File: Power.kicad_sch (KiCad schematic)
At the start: 23 parts, among them IC1 SC4216HSETRT, J4 Conn_01x03, J5 Conn_01x02, U8 TPS62933P

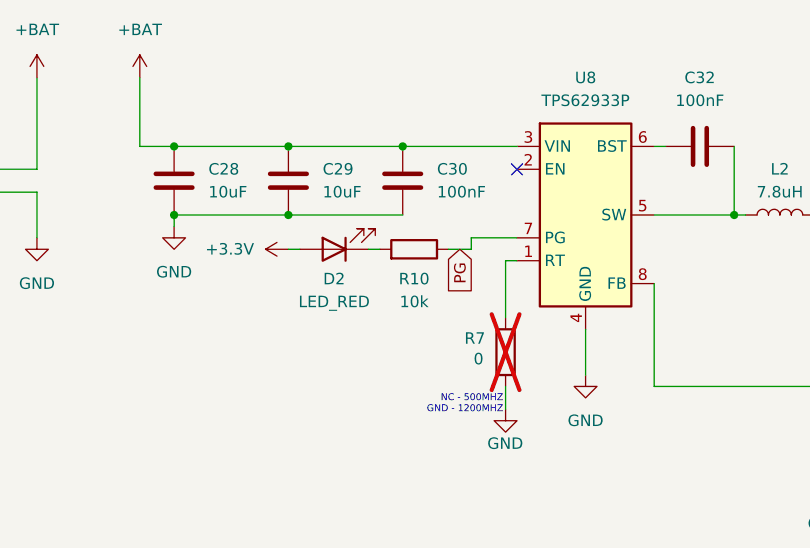
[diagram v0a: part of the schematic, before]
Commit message: "Update KiRA Flight Computer schematic and PCB files"
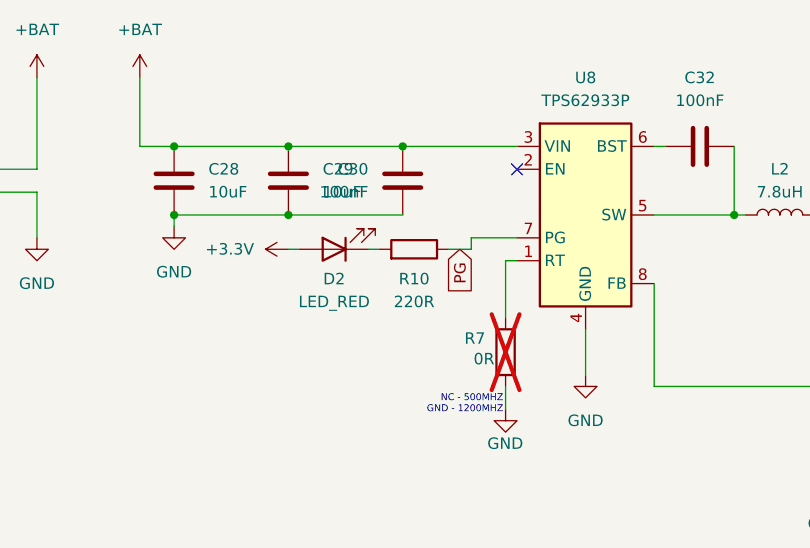
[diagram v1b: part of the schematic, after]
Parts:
- C28: footprint (none) -> Capacitor_SMD:C_1206_3216Metric; Source (none) -> https://www.lcsc.com/product-detail/C89632.html
- C29, C34, C35: footprint (none) -> Capacitor_SMD:C_1206_3216Metric
- C30: footprint (none) -> Capacitor_SMD:C_0603_1608Metric; Source (none) -> https://www.lcsc.com/product-detail/C1591.html
- C31: footprint (none) -> Capacitor_SMD:C_1210_3225Metric
- C32, C36: footprint (none) -> Capacitor_SMD:C_0603_1608Metric
- C33: footprint (none) -> Capacitor_SMD:C_0603_1608Metric; Source (none) -> https://www.lcsc.com/product-detail/C69335.html
- D2, D3: footprint (none) -> LED_SMD:LED_0603_1608Metric
- IC1: footprint SOIC127P600X175-9N -> dep:SOIC127P600X175-9N
- J4: footprint (none) -> Connector_PinSocket_2.54mm:PinSocket_1x03_P2.54mm_Vertical
- J5: footprint (none) -> Connector_AMASS:AMASS_XT30U-F_1x02_P5.0mm_Vertical
- L2: footprint (none) -> dep:Inductor 60A782C
- R10: value 10k -> 220R; footprint (none) -> Resistor_SMD:R_0402_1005Metric
- R11: footprint (none) -> Resistor_SMD:R_0402_1005Metric
- R12, R8: footprint (none) -> Resistor_SMD:R_0805_2012Metric
- R13, R9: footprint (none) -> Resistor_SMD:R_0603_1608Metric
- R7: value 0 -> 0R; footprint (none) -> Resistor_SMD:R_0603_1608Metric
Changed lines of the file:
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@@
 			)
 		)
-		(property "Footprint" ""
+		(property "Footprint" "LED_SMD:LED_0603_1608Metric"
 			(at 228.6 87.63 0)
 			(effects
@@
 			)
 		)
-		(property "Footprint" ""
+		(property "Footprint" "Connector_AMASS:AMASS_XT30U-F_1x02_P5.0mm_Vertical"
 			(at 21.59 78.74 0)
 			(effects
@@
 			)
 		)
-		(property "Footprint" ""
+		(property "Footprint" "Connector_PinSocket_2.54mm:PinSocket_1x03_P2.54mm_Vertical"
 			(at 200.66 81.28 0)
 			(effects
@@
 			)
 		)
-		(property "Footprint" ""
+		(property "Footprint" "Resistor_SMD:R_0805_2012Metric"
 			(at 106.172 135.89 90)
 			(effects
@@
 			)
 		)
-		(property "Footprint" ""
+		(property "Footprint" "Capacitor_SMD:C_1210_3225Metric"
 			(at 138.1252 96.52 0)
 			(effects
@@
 			)
 		)
-		(property "Footprint" ""
+		(property "Footprint" "Resistor_SMD:R_0603_1608Metric"
 			(at 106.172 146.05 90)
 			(effects
@@
 			)
 		)
-		(property "Footprint" ""
+		(property "Footprint" "dep:Inductor 60A782C"
 			(at 119.38 81.28 0)
 			(effects
@@
 			)
 		)
-		(property "Footprint" ""
+		(property "Footprint" "Capacitor_SMD:C_1206_3216Metric"
 			(at 53.0352 81.28 0)
 			(effects
@@
 			)
 		)
+		(property "Source" "https://www.lcsc.com/product-detail/C89632.html"
+			(at 52.07 77.47 0)
+			(effects
+				(font
+					(size 1.27 1.27)
+				)
+				(hide yes)
+			)
+		)
 		(pin "1"
 		)
@@
 			)
 		)
-		(property "Footprint" ""
+		(property "Footprint" "LED_SMD:LED_0603_1608Metric"
 			(at 69.85 85.09 0)
 			(effects
@@
 			)
 		)
-		(property "Footprint" "SOIC127P600X175-9N"
+		(property "Footprint" "dep:SOIC127P600X175-9N"
 			(at 87.63 230.81 0)
 			(effects
@@
 			)
 		)
-		(property "Footprint" ""
+		(property "Footprint" "Resistor_SMD:R_0603_1608Metric"
 			(at 122.682 105.41 90)
 			(effects
@@
 			)
 		)
-		(property "Footprint" ""
+		(property "Footprint" "Capacitor_SMD:C_1206_3216Metric"
 			(at 40.3352 148.59 0)
 			(effects
@@
 			)
 		)
-		(property "Footprint" ""
+		(property "Footprint" "Capacitor_SMD:C_0603_1608Metric"
 			(at 114.3 72.6948 0)
 			(effects
@@
 			)
 		)
-		(property "Footprint" ""
+		(property "Footprint" "Capacitor_SMD:C_0603_1608Metric"
 			(at 51.7652 148.59 0)
 			(effects
@@
 		)
 		(property "Description" "Unpolarized capacitor"
+			(at 50.8 144.78 0)
+			(effects
+				(font
+					(size 1.27 1.27)
+				)
+				(hide yes)
+			)
+		)
+		(property "Source" "https://www.lcsc.com/product-detail/C69335.html"
 			(at 50.8 144.78 0)
 			(effects
@@
 			)
 		)
-		(property "Footprint" ""
+		(property "Footprint" "Resistor_SMD:R_0402_1005Metric"
 			(at 226.822 95.25 90)
 			(effects
@@
 			)
 		)
-		(property "Value" "0"
+		(property "Value" "0R"
 			(at 85.344 97.282 0)
 			(effects
@@
 			)
 		)
-		(property "Footprint" ""
+		(property "Footprint" "Resistor_SMD:R_0603_1608Metric"
 			(at 87.122 96.52 90)
 			(effects
@@
 			)
 		)
-		(property "Footprint" ""
+		(property "Footprint" "Capacitor_SMD:C_1206_3216Metric"
 			(at 65.7352 81.28 0)
 			(effects
@@
 			)
 		)
-		(property "Footprint" ""
+		(property "Footprint" "Capacitor_SMD:C_0603_1608Metric"
 			(at 136.8552 149.86 0)
 			(effects
@@
 			)
 		)
-		(property "Footprint" ""
+		(property "Footprint" "Resistor_SMD:R_0805_2012Metric"
 			(at 122.682 92.71 90)
 			(effects
@@
 		(lib_id "Device:C")
 		(at 77.47 77.47 0)
-		(unit 1)
-		(exclude_from_sim no)
-		(in_bom yes)
-		(on_board yes)
-		(dnp no)
-		(fields_autoplaced yes)
+		(mirror y)
+		(unit 1)
+		(exclude_from_sim no)
+		(in_bom yes)
+		(on_board yes)
+		(dnp no)
 		(property "Reference" "C30"
-			(at 81.28 76.1999 0)
+			(at 73.66 76.1999 0)
 			(effects
 				(font
@@
 		)
 		(property "Value" "100nF"
-			(at 81.28 78.7399 0)
-			(effects
-				(font
-					(size 1.27 1.27)
-				)
-				(justify left)
-			)
-		)
-		(property "Footprint" ""
-			(at 78.4352 81.28 0)
+			(at 73.66 78.7399 0)
+			(effects
+				(font
+					(size 1.27 1.27)
+				)
+				(justify left)
+			)
+		)
+		(property "Footprint" "Capacitor_SMD:C_0603_1608Metric"
+			(at 76.5048 81.28 0)
 			(effects
 				(font
@@
 		)
 		(property "Description" "Unpolarized capacitor"
+			(at 77.47 77.47 0)
+			(effects
+				(font
+					(size 1.27 1.27)
+				)
+				(hide yes)
+			)
+		)
+		(property "Source" "https://www.lcsc.com/product-detail/C1591.html"
 			(at 77.47 77.47 0)
 			(effects
@@
 			)
 		)
-		(property "Footprint" ""
+		(property "Footprint" "Capacitor_SMD:C_1206_3216Metric"
 			(at 125.4252 149.86 0)
 			(effects
@@
 			)
 		)
-		(property "Value" "10k"
+		(property "Value" "220R"
 			(at 78.74 90.932 90)
 			(effects
@@
 			)
 		)
-		(property "Footprint" ""
+		(property "Footprint" "Resistor_SMD:R_0402_1005Metric"
 			(at 78.74 86.868 90)
 			(effects

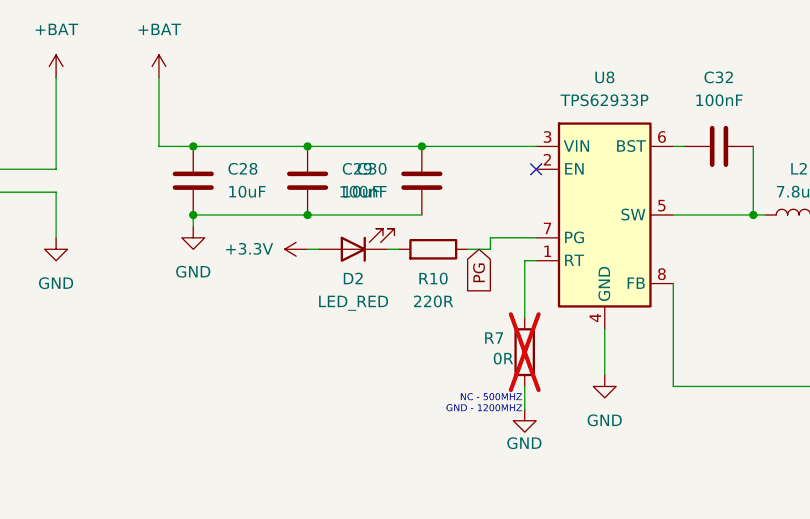
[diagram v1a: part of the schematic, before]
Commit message: Update PCB
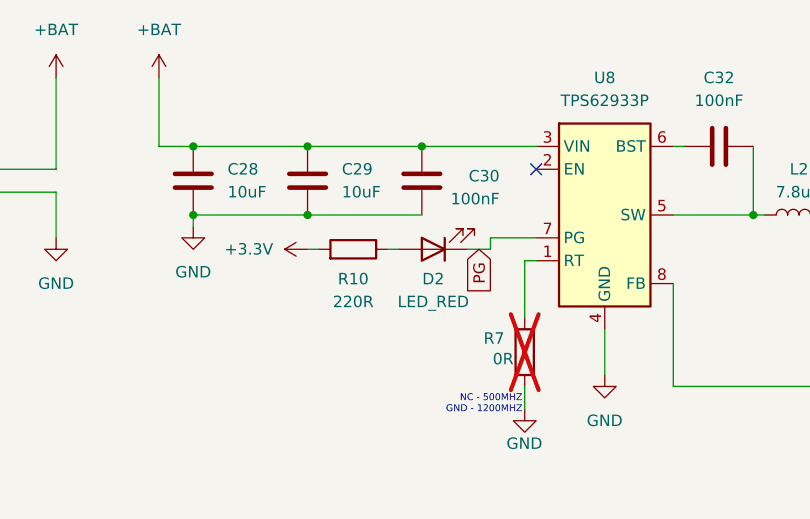
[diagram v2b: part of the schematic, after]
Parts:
- L2: footprint dep:Inductor 60A782C -> Inductor_SMD:L_APV_APH1050
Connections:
- net +3.3V: now also R10.2; no longer D2.2 (A)
- net PG: now also D2.1 (K); no longer R10.1
- new net: D2.2 (A), R10.1
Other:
- moved on the sheet: D2, R10
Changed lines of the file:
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@@
 			)
 		)
-		(property "Footprint" "dep:Inductor 60A782C"
+		(property "Footprint" "Inductor_SMD:L_APV_APH1050"
 			(at 119.38 81.28 0)
 			(effects
@@
 	(symbol
 		(lib_id "Device:LED")
-		(at 69.85 85.09 180)
+		(at 78.74 85.09 180)
 		(unit 1)
 		(exclude_from_sim no)
@@
 		(dnp no)
 		(property "Reference" "D2"
-			(at 69.85 88.392 0)
+			(at 78.74 88.392 0)
 			(effects
 				(font
@@
 		)
 		(property "Value" "LED_RED"
-			(at 69.85 90.932 0)
+			(at 78.74 90.932 0)
 			(effects
 				(font
@@
 		)
 		(property "Footprint" "LED_SMD:LED_0603_1608Metric"
-			(at 69.85 85.09 0)
+			(at 78.74 85.09 0)
 			(effects
 				(font
@@
 		)
 		(property "Datasheet" "~"
-			(at 69.85 85.09 0)
+			(at 78.74 85.09 0)
 			(effects
 				(font
@@
 		)
 		(property "Description" "Light emitting diode"
-			(at 69.85 85.09 0)
+			(at 78.74 85.09 0)
 			(effects
 				(font
@@
 		)
 		(property "Sim.Pins" "1=K 2=A"
-			(at 69.85 85.09 0)
+			(at 78.74 85.09 0)
 			(effects
 				(font
@@
 		(on_board yes)
 		(dnp no)
-		(fields_autoplaced yes)
 		(property "Reference" "C29"
 			(at 68.58 76.1999 0)
@@
 		(on_board yes)
 		(dnp no)
-		(fields_autoplaced yes)
 		(property "Reference" "C36"
 			(at 139.7 144.7799 0)
@@
 		(dnp no)
 		(property "Reference" "C30"
-			(at 73.66 76.1999 0)
+			(at 86.106 76.962 0)
 			(effects
 				(font
@@
 		)
 		(property "Value" "100nF"
-			(at 73.66 78.7399 0)
+			(at 86.106 79.502 0)
 			(effects
 				(font
@@
 	(symbol
 		(lib_id "Device:R")
-		(at 78.74 85.09 270)
+		(at 69.85 85.09 270)
 		(mirror x)
 		(unit 1)
@@
 		(dnp no)
 		(property "Reference" "R10"
-			(at 78.74 88.392 90)
+			(at 69.85 88.392 90)
 			(effects
 				(font
@@
 		)
 		(property "Value" "220R"
-			(at 78.74 90.932 90)
+			(at 69.85 90.932 90)
 			(effects
 				(font
@@
 		)
 		(property "Footprint" "Resistor_SMD:R_0402_1005Metric"
-			(at 78.74 86.868 90)
+			(at 69.85 86.868 90)
 			(effects
 				(font
@@
 		)
 		(property "Datasheet" "~"
-			(at 78.74 85.09 0)
+			(at 69.85 85.09 0)
 			(effects
 				(font
@@
 		)
 		(property "Description" "Resistor"
-			(at 78.74 85.09 0)
-			(effects
-				(font
+			(at 69.85 85.09 0)
+			(effects
+				(font
